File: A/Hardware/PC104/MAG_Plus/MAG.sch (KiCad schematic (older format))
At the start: 2 parts, among them J7 Conn_01x04_Male, J8 Conn_01x04_Male

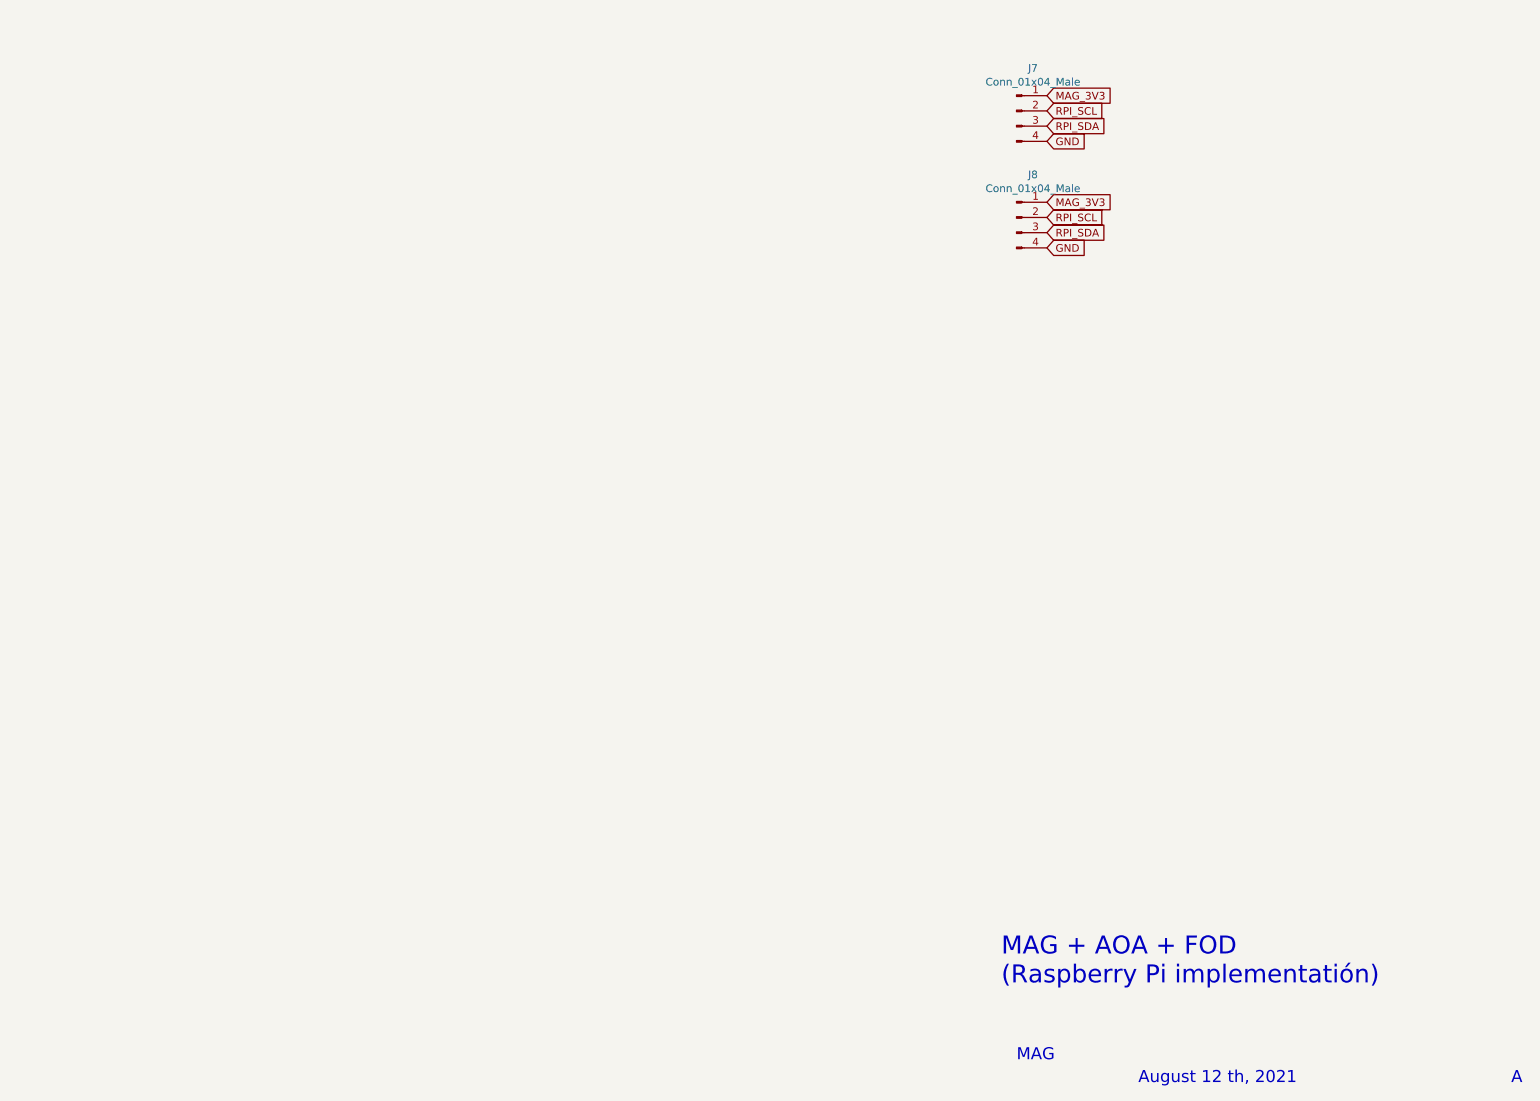
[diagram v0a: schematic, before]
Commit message: PCB update
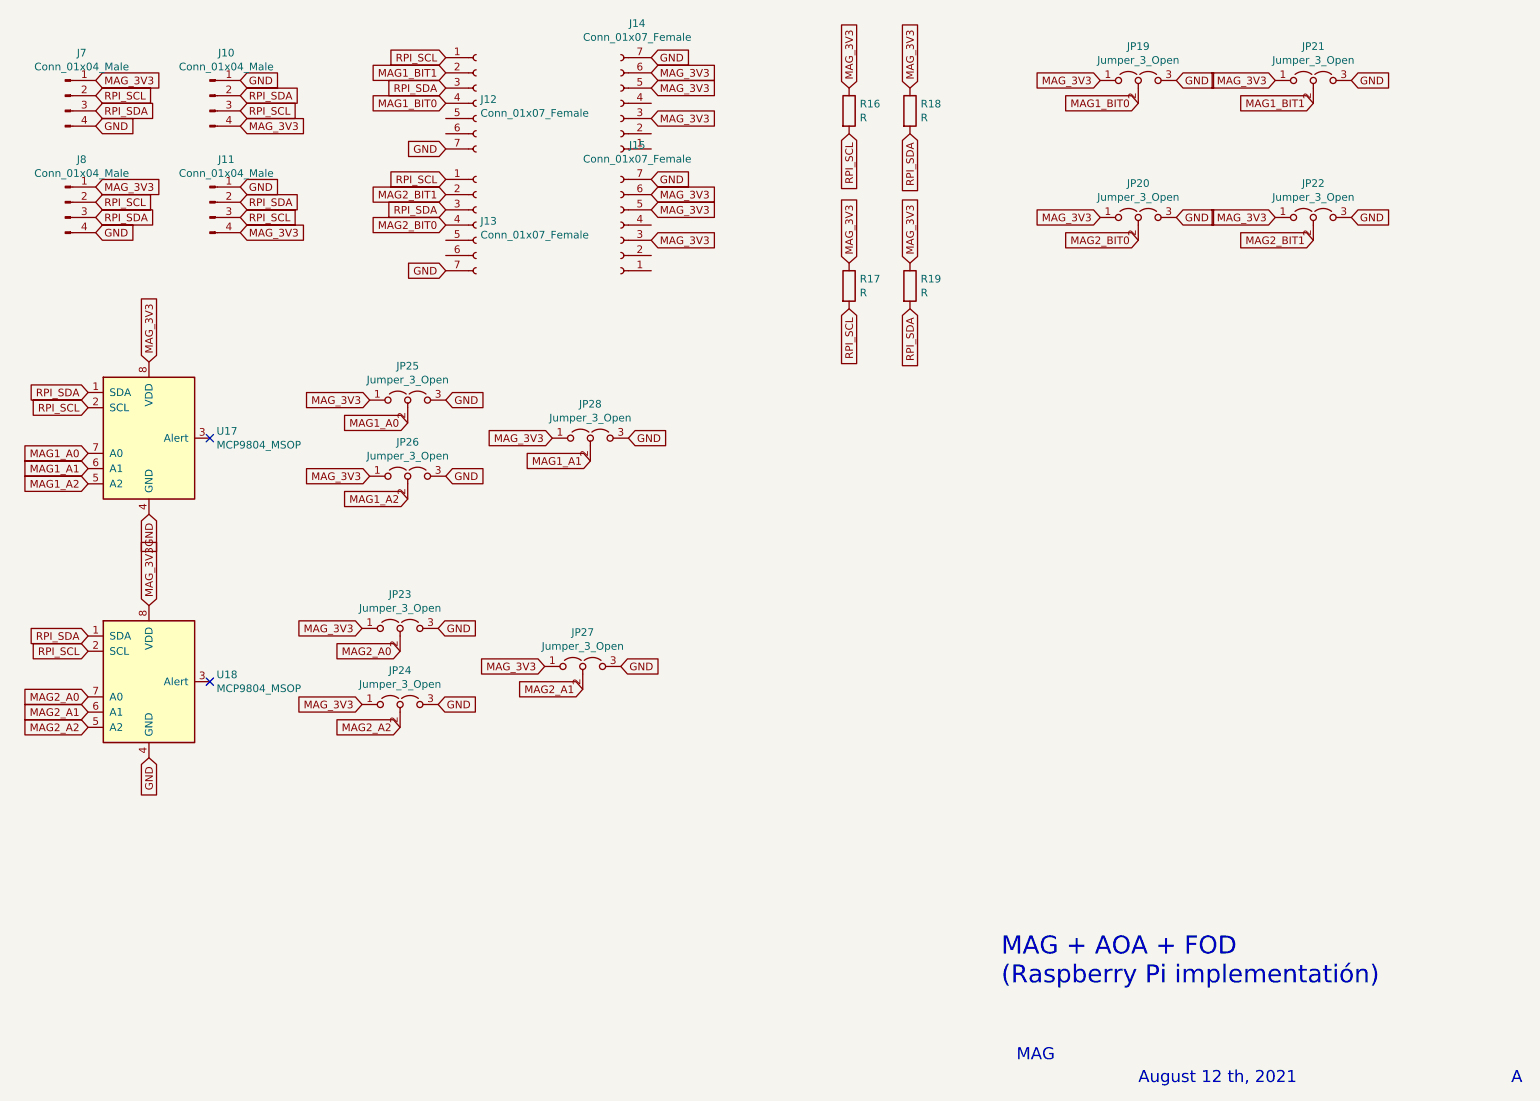
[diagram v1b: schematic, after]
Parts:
- added J10, J11: Conn_01x04_Male, Connectors_Molex:Molex_PicoBlade_53398-0471_04x1.25mm_Straight, symbol Connector:Conn_01x04_Male
- added J12, J14: Conn_01x07_Female, Pin_Headers:Pin_Header_Straight_1x07_Pitch2.54mm_SMD_Pin1Left, symbol Connector:Conn_01x07_Female
- added J13, J15: Conn_01x07_Female, Pin_Headers:Pin_Header_Straight_1x07_Pitch2.54mm_SMD_Pin1Right, symbol Connector:Conn_01x07_Female
- added JP19, JP20, JP21, JP22, JP23, JP24, JP25, JP26, JP27, JP28: Jumper_3_Open, Jumper:SolderJumper-3_P1.3mm_Open_RoundedPad1.0x1.5mm, symbol Jumper:Jumper_3_Open
- added R16, R17, R18, R19: R, Resistors_SMD:R_0402, symbol Device:R
- added U17, U18: MCP9804_MSOP, Housings_SSOP:MSOP-8_3x3mm_Pitch0.65mm, symbol Sensor_Temperature:MCP9804_MSOP
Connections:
- net GND: now also J10.1 (Pin_1), J11.1 (Pin_1), J12.7 (Pin_7), J13.7 (Pin_7), J14.7 (Pin_7), J15.7 (Pin_7), JP19.3 (B), JP20.3 (B), JP21.3 (B), JP22.3 (B), JP23.3 (B), JP24.3 (B), JP25.3 (B), JP26.3 (B), JP27.3 (B), JP28.3 (B), U17.4 (GND), U18.4 (GND)
- net MAG_3V3: now also J10.4 (Pin_4), J11.4 (Pin_4), J14.3 (Pin_3), J14.5 (Pin_5), J14.6 (Pin_6), J15.3 (Pin_3), J15.5 (Pin_5), J15.6 (Pin_6), JP19.1 (A), JP20.1 (A), JP21.1 (A), JP22.1 (A), JP23.1 (A), JP24.1 (A), JP25.1 (A), JP26.1 (A), JP27.1 (A), JP28.1 (A), R16.1, R17.1, R18.1, R19.1, U17.8 (VDD), U18.8 (VDD)
- net RPI_SCL: now also J10.3 (Pin_3), J11.3 (Pin_3), J12.1 (Pin_1), J13.1 (Pin_1), R16.2, R17.2, U17.2 (SCL), U18.2 (SCL)
- net RPI_SDA: now also J10.2 (Pin_2), J11.2 (Pin_2), J12.3 (Pin_3), J13.3 (Pin_3), R18.2, R19.2, U17.1 (SDA), U18.1 (SDA)
- new net MAG1_A0: JP25.2 (C), U17.7 (A0)
- new net MAG1_A1: JP28.2 (C), U17.6 (A1)
- new net MAG1_A2: JP26.2 (C), U17.5 (A2)
- new net MAG1_BIT0: J12.4 (Pin_4), JP19.2 (C)
- new net MAG1_BIT1: J12.2 (Pin_2), JP21.2 (C)
- new net MAG2_A0: JP23.2 (C), U18.7 (A0)
- new net MAG2_A1: JP27.2 (C), U18.6 (A1)
- new net MAG2_A2: JP24.2 (C), U18.5 (A2)
- new net MAG2_BIT0: J13.4 (Pin_4), JP20.2 (C)
- new net MAG2_BIT1: J13.2 (Pin_2), JP22.2 (C)
- no-connect marks 0 -> 2
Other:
- moved on the sheet: J7, J8
